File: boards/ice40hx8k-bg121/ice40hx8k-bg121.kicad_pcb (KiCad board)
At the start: 4 copper layers, 22.9 x 48.3 mm, 60 parts, among them J1 Conn_01x16, J2 Conn_01x16, J3 Conn_02x06_Odd_Even, J4 Conn_02x06_Odd_Even, SW1 B3U-1000P, U1 AP7361C-33Y5-13, U2 AP7361C-12Y5-13, U3 iCE40HX8K-BG121(121-Ball_caBG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, U4 LE25U20AMB, U5 ASDMB-xxxMHz

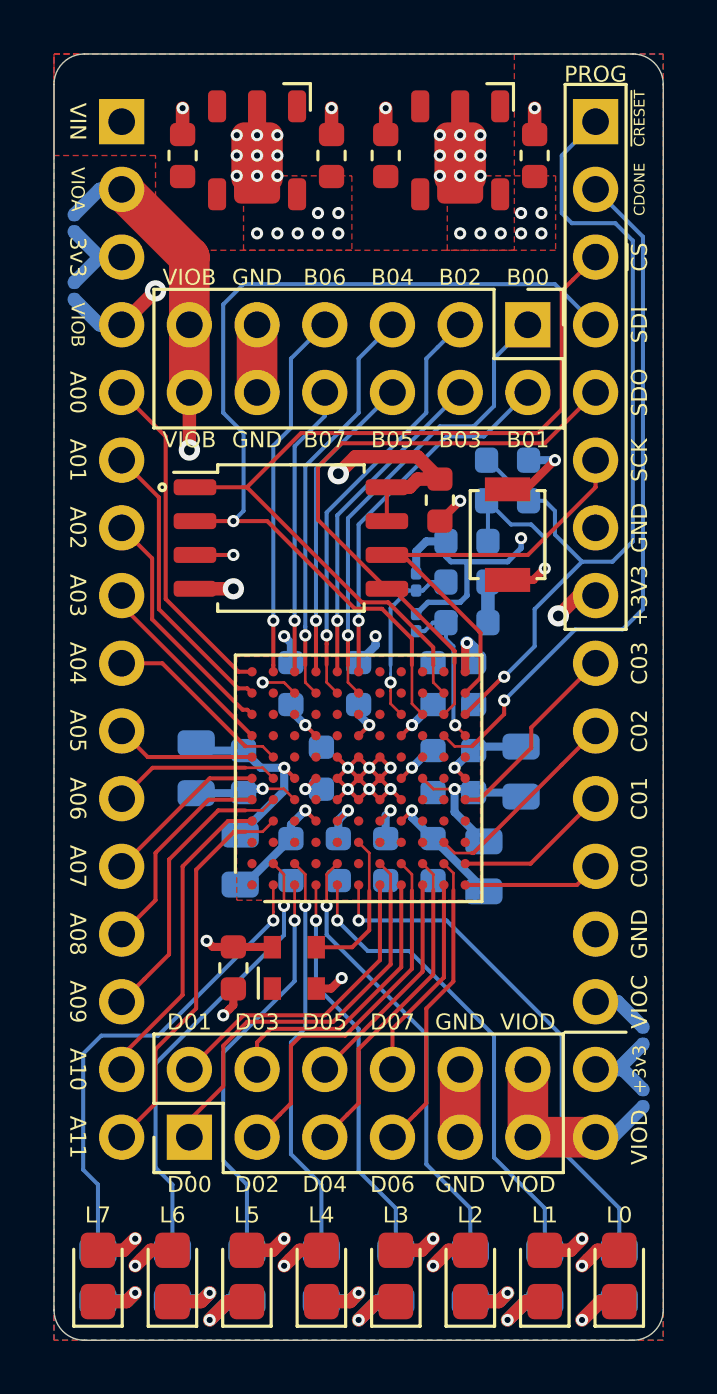
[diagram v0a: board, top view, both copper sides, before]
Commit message: Updated version info on backside of board.
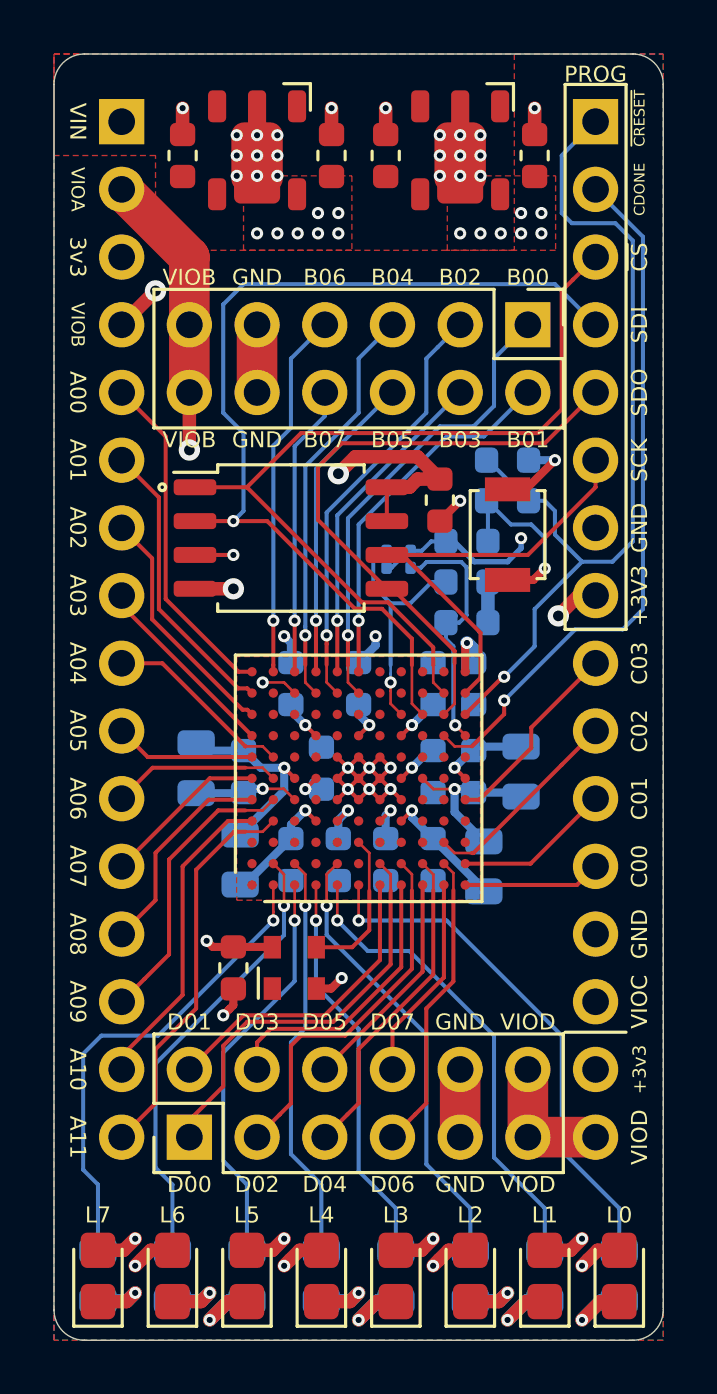
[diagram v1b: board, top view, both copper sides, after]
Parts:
- removed JP3: VCCIO_A, jkiv-library:J_NO_0201_0603Metric
- removed JP4: VCCIO_B, jkiv-library:J_NO_0201_0603Metric
- removed JP5: VCCIO_C, jkiv-library:J_NO_0201_0603Metric
- removed JP6: VCCIO_D, jkiv-library:J_NO_0201_0603Metric
- moved JP1 2.39 mm to (33.7, 34.2)
- moved JP2 1.40 mm to (32.8, 34.2), turned to 90 degrees
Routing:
- net +3V3: track 47.1 -> 36.1 mm
- net CBSEL0: track 5.84 -> 9.55 mm
- net CBSEL1: track 6.63 -> 9.35 mm
- net VCCIO_D: track 25.5 -> 23.3 mm
- net VCCIO_C: track 18.1 -> 15.9 mm
- net VCCIO_B: track 30.4 -> 28.3 mm
- net VCCIO_A: track 27.5 -> 25.4 mm
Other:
- board text added: "(cc) fourside.io"
- board text added: "ice40hx8k breakout 2020-04"
- board text removed: "fourside.io"
- board text removed: "ice40hx8k breakout 2020-03"
